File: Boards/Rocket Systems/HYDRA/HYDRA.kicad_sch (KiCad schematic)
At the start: 22 parts, among them IC1 NSVT30010MXV6T1G, IC2 BC846BLT1G, U1 VLMKG3400-GS08

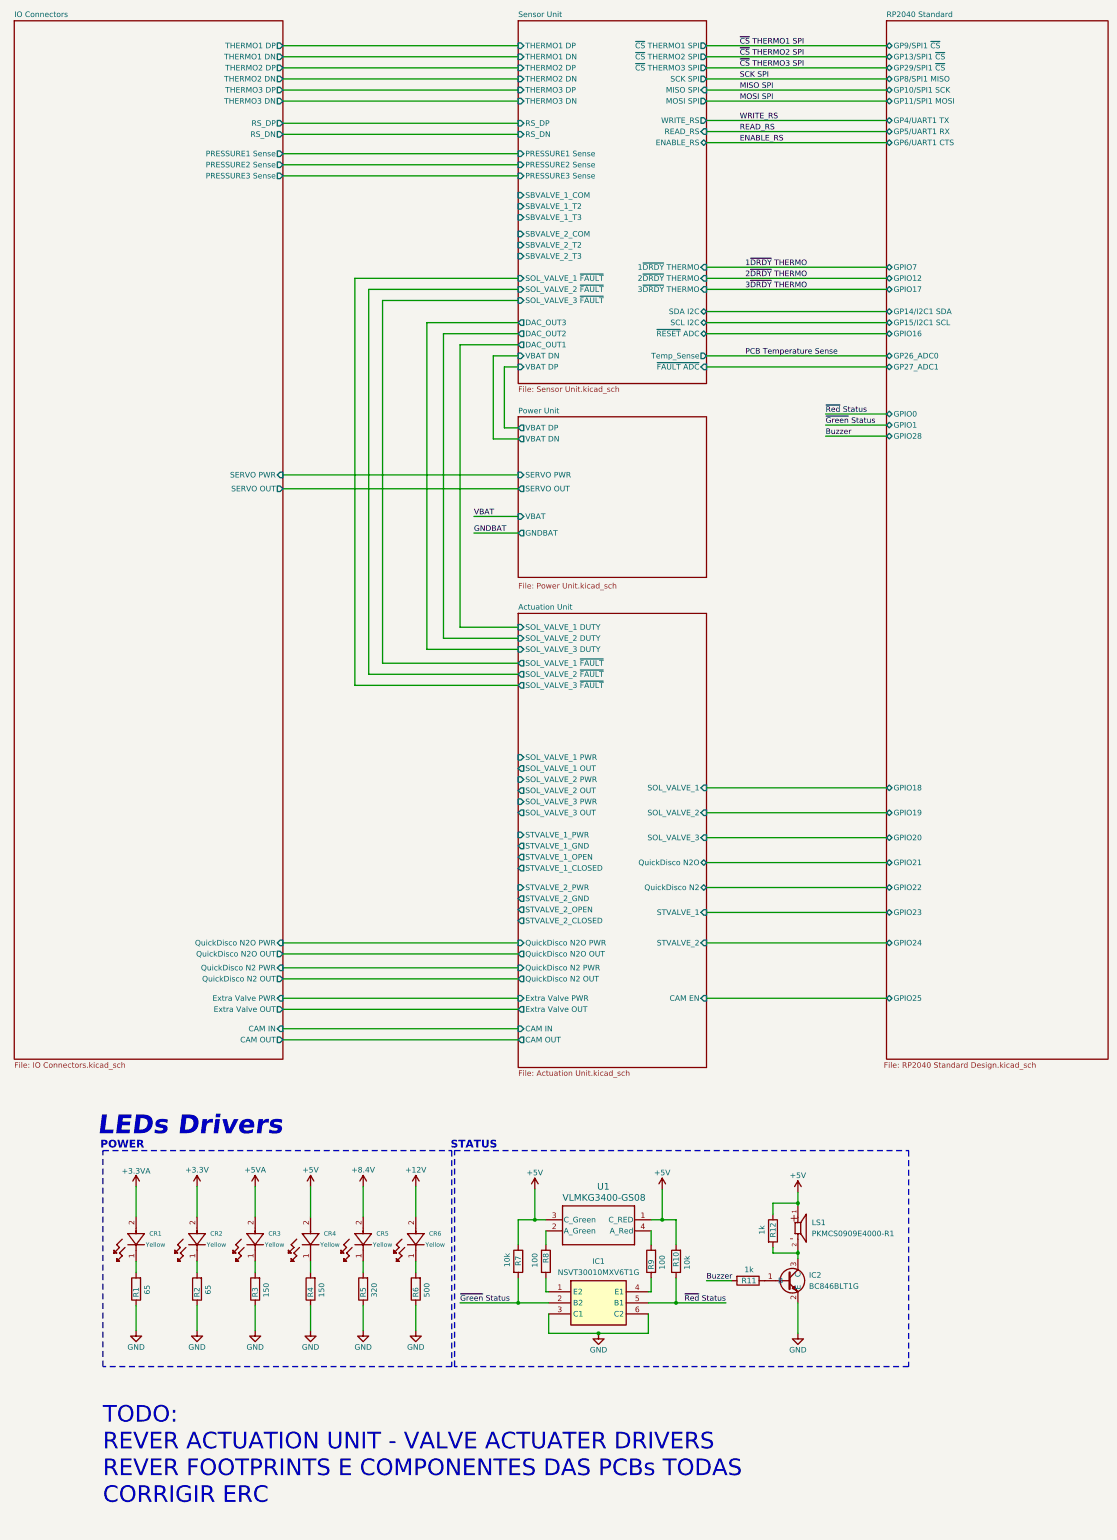
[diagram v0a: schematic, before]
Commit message: HYDRA Update - footprints and schematics
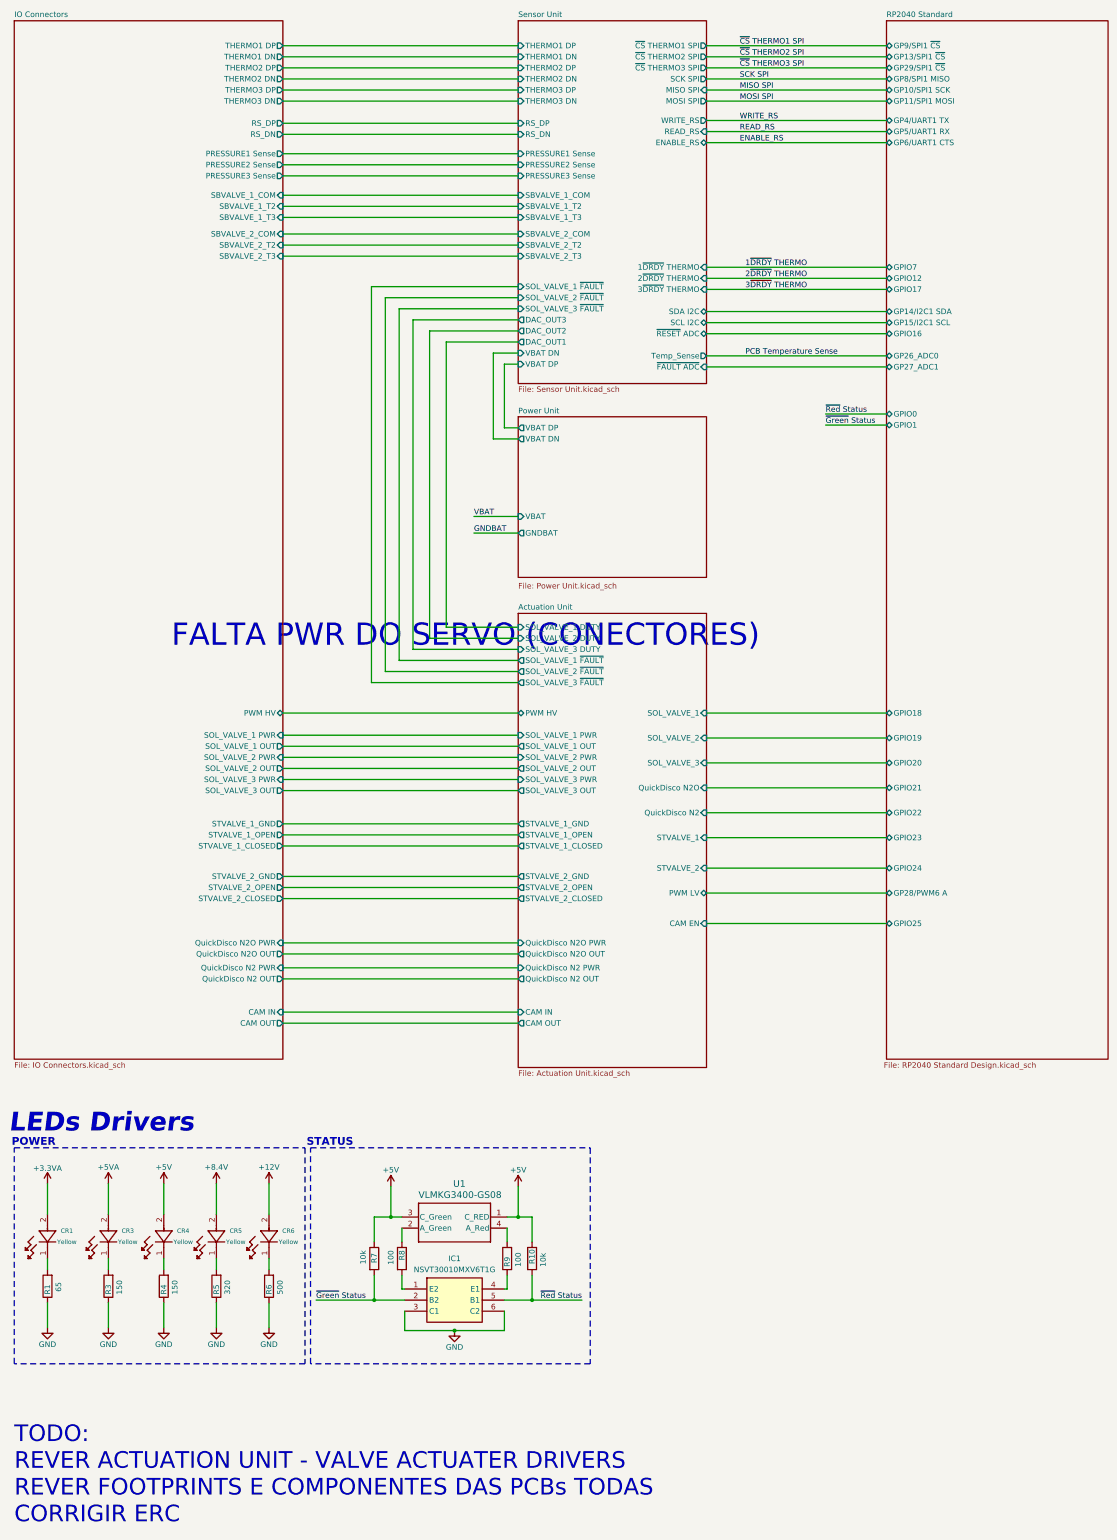
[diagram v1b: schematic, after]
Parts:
- removed CR2: VLMY1300-GS08, LED-Yellow_VLMY1300-GS08:LED_VISHAY_VLMX1300_VIS, symbol VLMY1300-GS08:VLMY1300-GS08
- removed IC2: BC846BLT1G, BJT NPN:SOT96P237X111-3N, symbol BC846BLT1G:BC846BLT1G
- removed LS1: PKMCS0909E4000-R1, PKMCS0909E4000-R1:SPKR_PKMCS0909E4000-R1, symbol PKMCS0909E4000-R1:PKMCS0909E4000-R1
- removed R11, R12: 1k, Resistor-0402:RES_0402, symbol Device:R
- removed R2: 65, Resistor-0402:RES_0402, symbol Device:R
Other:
- sheet Actuation Unit ports: added PWM HV, PWM LV; removed Extra Valve OUT, Extra Valve PWR, STVALVE_1_PWR, STVALVE_2_PWR
- sheet IO Connectors ports: added PWM HV, SBVALVE_1_COM, SBVALVE_1_T2, SBVALVE_1_T3, SBVALVE_2_COM, SBVALVE_2_T2, SBVALVE_2_T3, SOL_VALVE_1 OUT, SOL_VALVE_1 PWR, SOL_VALVE_2 OUT, SOL_VALVE_2 PWR, SOL_VALVE_3 OUT, SOL_VALVE_3 PWR, STVALVE_1_CLOSED, STVALVE_1_GND, STVALVE_1_OPEN, STVALVE_2_CLOSED, STVALVE_2_GND, STVALVE_2_OPEN; removed Extra Valve OUT, Extra Valve PWR, SERVO OUT, SERVO PWR
- sheet Power Unit ports: added none; removed SERVO OUT, SERVO PWR
- sheet RP2040 Standard ports: added GP28/PWM6 A; removed GPIO28
- note added: "FALTA PWR DO SERVO (CONECTORES)"
- moved on the sheet: CR1, CR3, CR4, CR5, CR6, IC1, R1, R10, R3, R4, R5, R6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
